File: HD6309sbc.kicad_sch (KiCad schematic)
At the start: 24 parts, among them J1 Conn_01x02_Male, J3 Conn_01x02_Male, U1 HD63C09, U11 74HC02, U12 74AHC1G08, U13 74HC21D, U14 74HC21D, U15 74HC21D, U4 UM61256FK, U6 28C256, U7 74HC04D, U8 74HC00D

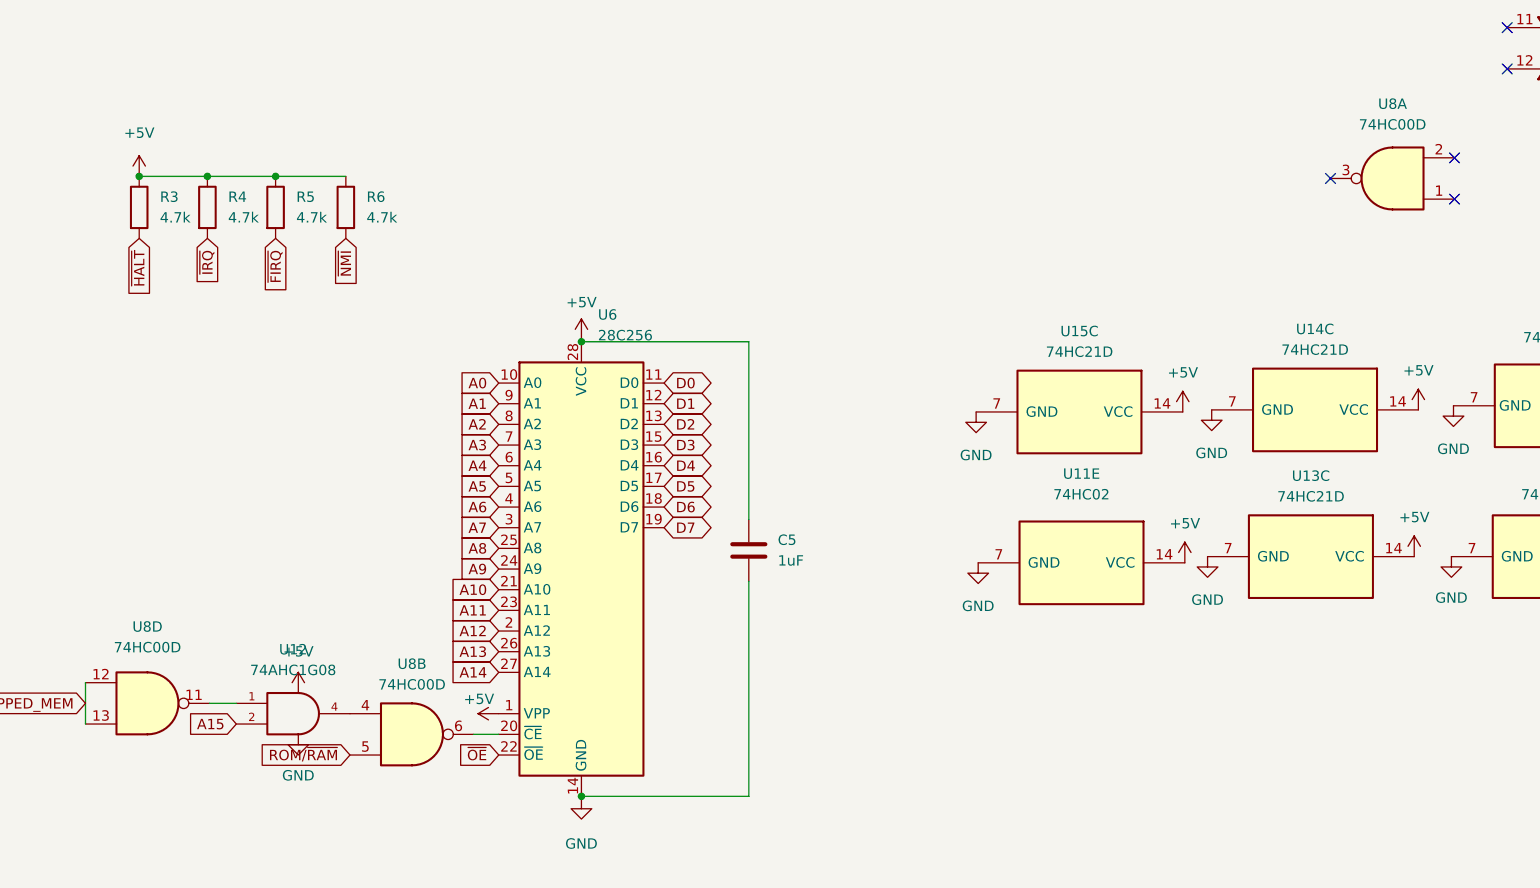
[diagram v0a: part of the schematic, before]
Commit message: convert to discrete clock
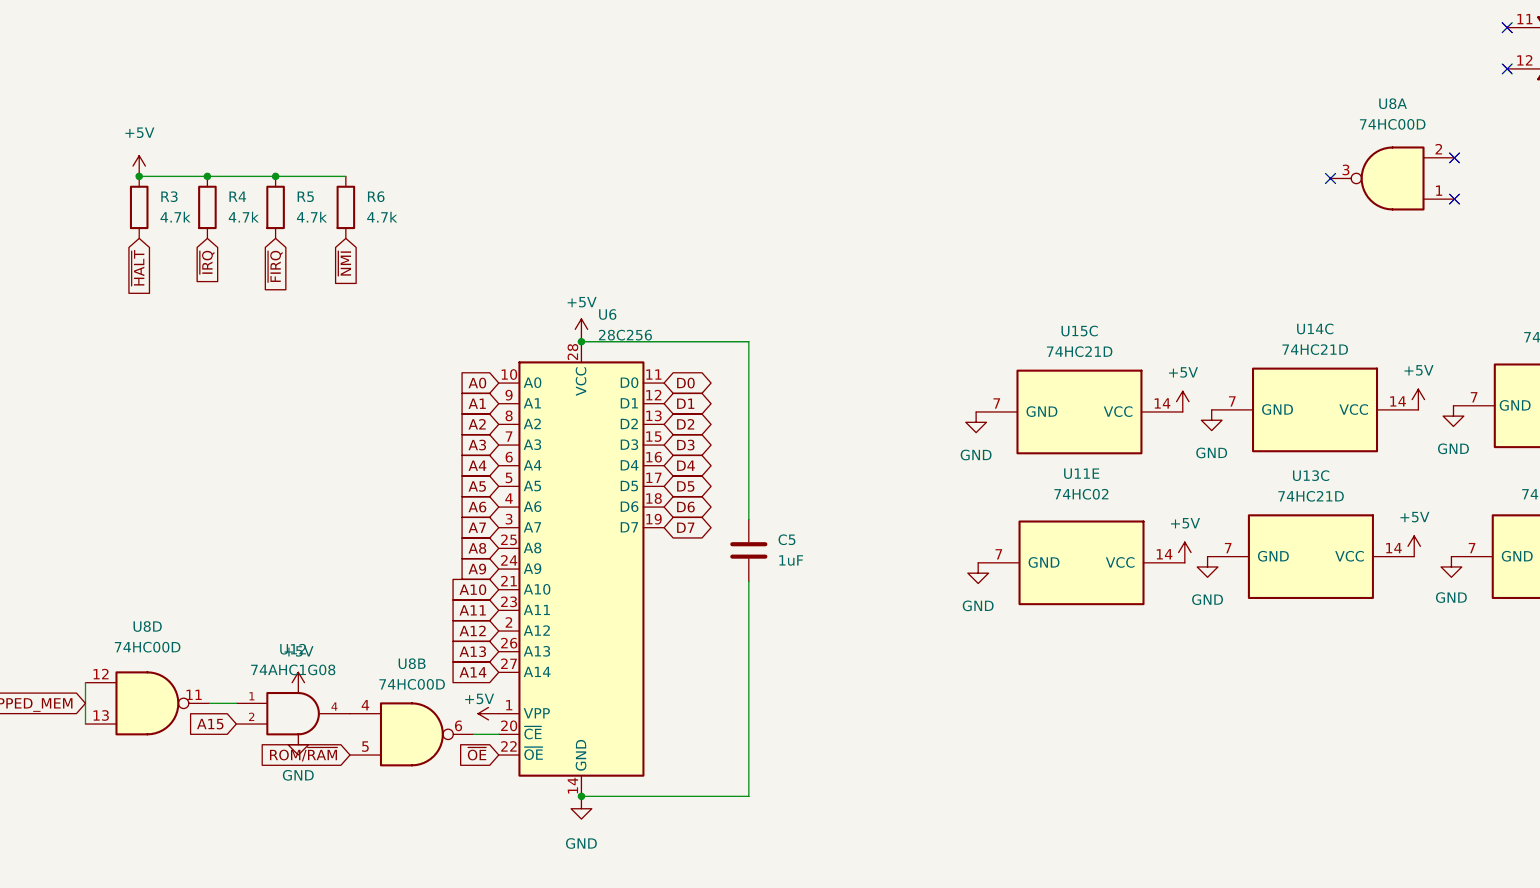
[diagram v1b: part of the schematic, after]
